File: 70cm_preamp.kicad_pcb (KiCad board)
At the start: 2 copper layers, 33.4 x 13.2 mm, 7 parts, among them J1 RF_IN, J2 RF_OUT, U1 SF2446E, U2 PGA-103+

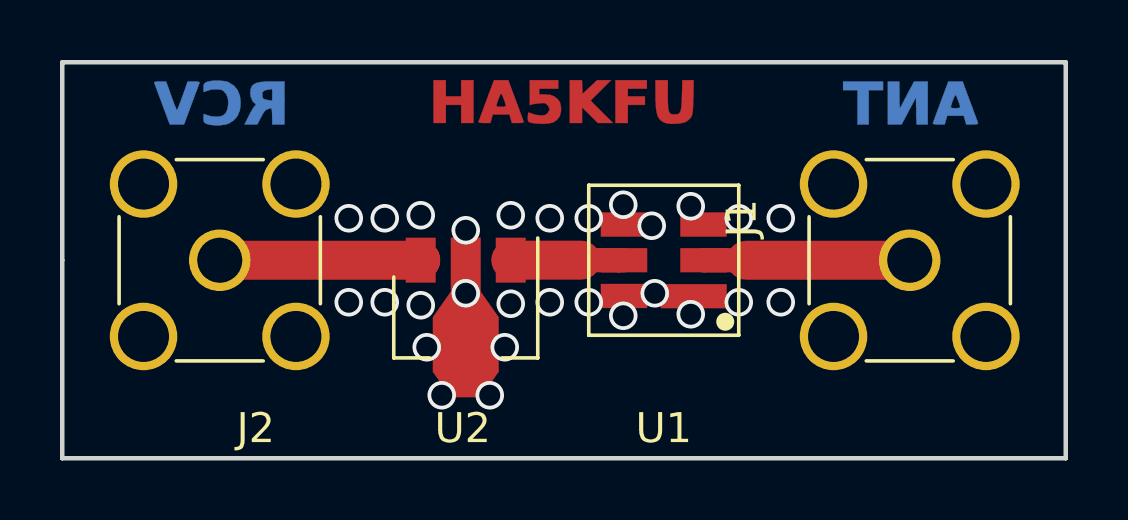
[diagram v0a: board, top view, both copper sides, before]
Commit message: viák
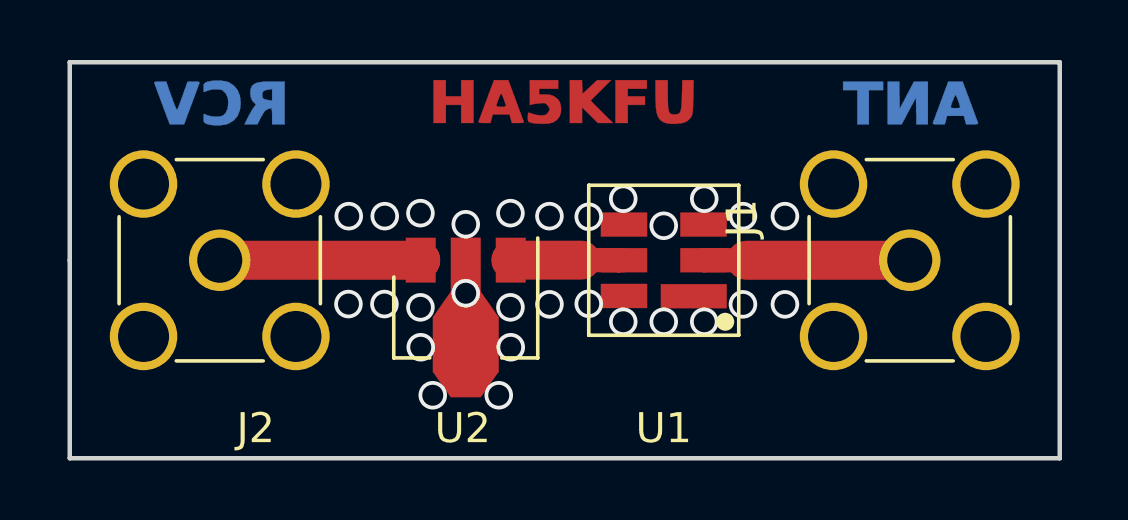
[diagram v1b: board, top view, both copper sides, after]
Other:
- board size 33.4 x 13.2 mm -> 33 x 13.2 mm
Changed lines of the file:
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@@
-(kicad_pcb (version 20171130) (host pcbnew 5.1.6-c6e7f7d~86~ubuntu19.10.1)
+(kicad_pcb (version 20171130) (host pcbnew 5.1.5+dfsg1-2build2)
   (general
     (thickness 1.6)
@@
     )
   )
-  (gr_line (start 42.35 43.4) (end 42.35 36.8) (layer Edge.Cuts) (width 0.15))
-  (gr_line (start 75.8 43.4) (end 42.35 43.4) (layer Edge.Cuts) (width 0.15))
-  (gr_line (start 75.8 30.2) (end 75.8 43.4) (layer Edge.Cuts) (width 0.15))
-  (gr_line (start 42.35 30.2) (end 75.8 30.2) (layer Edge.Cuts) (width 0.15))
-  (gr_line (start 42.35 36.8) (end 42.35 30.2) (layer Edge.Cuts) (width 0.15))
+  (gr_line (start 42.6 43.4) (end 42.6 36.8) (layer Edge.Cuts) (width 0.15))
+  (gr_line (start 75.6 43.4) (end 42.6 43.4) (layer Edge.Cuts) (width 0.15))
+  (gr_line (start 75.6 30.2) (end 75.6 43.4) (layer Edge.Cuts) (width 0.15))
+  (gr_line (start 42.6 30.2) (end 75.6 30.2) (layer Edge.Cuts) (width 0.15))
+  (gr_line (start 42.6 36.8) (end 42.6 30.2) (layer Edge.Cuts) (width 0.15))
   (segment (start 54.2965 36.8) (end 54.3 36.7965) (width 1.3) (layer F.Cu) (net 1))
   (segment (start 47.6 36.8) (end 54.2965 36.8) (width 1.3) (layer F.Cu) (net 1))
-  (via (at 54.3 35.3) (size 0.95) (drill 0.7) (layers F.Cu B.Cu) (net 2))
-  (via (at 53.1 35.4) (size 0.95) (drill 0.7) (layers F.Cu B.Cu) (net 2))
-  (via (at 53.1 38.2) (size 0.95) (drill 0.7) (layers F.Cu B.Cu) (net 2))
-  (via (at 54.3 38.3) (size 0.95) (drill 0.7) (layers F.Cu B.Cu) (net 2))
-  (via (at 57.3 35.3) (size 0.95) (drill 0.7) (layers F.Cu B.Cu) (net 2))
-  (via (at 57.3 38.25) (size 0.95) (drill 0.7) (layers F.Cu B.Cu) (net 2))
-  (via (at 62.1 37.9) (size 0.95) (drill 0.7) (layers F.Cu B.Cu) (net 2))
-  (via (at 62 35.65) (size 0.95) (drill 0.7) (layers F.Cu B.Cu) (net 2))
-  (via (at 63.3 35) (size 0.95) (drill 0.7) (layers F.Cu B.Cu) (net 2))
-  (via (at 63.3 38.6) (size 0.95) (drill 0.7) (layers F.Cu B.Cu) (net 2))
-  (via (at 59.9 38.2) (size 0.95) (drill 0.7) (layers F.Cu B.Cu) (net 2))
-  (via (at 59.9 35.4) (size 0.95) (drill 0.7) (layers F.Cu B.Cu) (net 2))
-  (via (at 58.6 38.2) (size 0.95) (drill 0.7) (layers F.Cu B.Cu) (net 2))
-  (via (at 51.9 38.2) (size 0.95) (drill 0.7) (layers F.Cu B.Cu) (net 2))
-  (via (at 51.9 35.4) (size 0.95) (drill 0.7) (layers F.Cu B.Cu) (net 2))
+  (via (at 54.29 35.23) (size 0.95) (drill 0.7) (layers F.Cu B.Cu) (net 2))
+  (via (at 53.1 35.33) (size 0.95) (drill 0.7) (layers F.Cu B.Cu) (net 2))
+  (via (at 53.09 38.26) (size 0.95) (drill 0.7) (layers F.Cu B.Cu) (net 2))
+  (via (at 54.29 38.37) (size 0.95) (drill 0.7) (layers F.Cu B.Cu) (net 2))
+  (via (at 57.29 35.23) (size 0.95) (drill 0.7) (layers F.Cu B.Cu) (net 2))
+  (via (at 57.29 38.37) (size 0.95) (drill 0.7) (layers F.Cu B.Cu) (net 2))
+  (via (at 62.4 35.65) (size 0.95) (drill 0.7) (layers F.Cu B.Cu) (net 2))
+  (via (at 63.75 34.75) (size 0.95) (drill 0.7) (layers F.Cu B.Cu) (net 2))
+  (via (at 63.75 38.85) (size 0.95) (drill 0.7) (layers F.Cu B.Cu) (net 2))
+  (via (at 59.9 38.25) (size 0.95) (drill 0.7) (layers F.Cu B.Cu) (net 2))
+  (via (at 59.9 35.35) (size 0.95) (drill 0.7) (layers F.Cu B.Cu) (net 2))
+  (via (at 58.59 38.27) (size 0.95) (drill 0.7) (layers F.Cu B.Cu) (net 2))
+  (via (at 51.89 38.26) (size 0.95) (drill 0.7) (layers F.Cu B.Cu) (net 2))
+  (via (at 51.9 35.33) (size 0.95) (drill 0.7) (layers F.Cu B.Cu) (net 2))
   (via (at 55.8 37.9) (size 0.95) (drill 0.7) (layers F.Cu B.Cu) (net 2))
-  (via (at 54.5 39.7) (size 0.95) (drill 0.7) (layers F.Cu B.Cu) (net 2))
-  (via (at 57.1 39.7) (size 0.95) (drill 0.7) (layers F.Cu B.Cu) (net 2))
-  (via (at 55 41.3) (size 0.95) (drill 0.7) (layers F.Cu B.Cu) (net 2))
-  (via (at 56.6 41.3) (size 0.95) (drill 0.7) (layers F.Cu B.Cu) (net 2))
-  (via (at 61.05 38.65) (size 0.95) (drill 0.7) (layers F.Cu B.Cu) (net 2))
-  (via (at 61.05 34.95) (size 0.95) (drill 0.7) (layers F.Cu B.Cu) (net 2))
-  (via (at 55.8 35.8) (size 0.95) (drill 0.7) (layers F.Cu B.Cu) (net 2))
-  (via (at 58.6 35.4) (size 0.95) (drill 0.7) (layers F.Cu B.Cu) (net 2))
-  (via (at 64.9 38.2) (size 0.95) (drill 0.7) (layers F.Cu B.Cu) (net 2))
-  (via (at 64.9 35.4) (size 0.95) (drill 0.7) (layers F.Cu B.Cu) (net 2))
-  (via (at 66.3 35.4) (size 0.95) (drill 0.7) (layers F.Cu B.Cu) (net 2))
-  (via (at 66.3 38.2) (size 0.95) (drill 0.7) (layers F.Cu B.Cu) (net 2))
+  (via (at 54.3 39.7) (size 0.95) (drill 0.7) (layers F.Cu B.Cu) (net 2))
+  (via (at 57.3 39.7) (size 0.95) (drill 0.7) (layers F.Cu B.Cu) (net 2))
+  (via (at 54.7 41.3) (size 0.95) (drill 0.7) (layers F.Cu B.Cu) (net 2))
+  (via (at 56.9 41.3) (size 0.95) (drill 0.7) (layers F.Cu B.Cu) (net 2))
+  (via (at 61.05 38.85) (size 0.95) (drill 0.7) (layers F.Cu B.Cu) (net 2))
+  (via (at 61.05 34.75) (size 0.95) (drill 0.7) (layers F.Cu B.Cu) (net 2))
+  (via (at 55.8 35.6) (size 0.95) (drill 0.7) (layers F.Cu B.Cu) (net 2))
+  (via (at 58.59 35.33) (size 0.95) (drill 0.7) (layers F.Cu B.Cu) (net 2))
+  (via (at 65.04 38.27) (size 0.95) (drill 0.7) (layers F.Cu B.Cu) (net 2))
+  (via (at 65.04 35.33) (size 0.95) (drill 0.7) (layers F.Cu B.Cu) (net 2))
+  (via (at 66.44 35.33) (size 0.95) (drill 0.7) (layers F.Cu B.Cu) (net 2))
+  (via (at 66.44 38.27) (size 0.95) (drill 0.7) (layers F.Cu B.Cu) (net 2))
+  (via (at 62.4 38.85) (size 0.95) (drill 0.7) (layers F.Cu B.Cu) (net 2))
   (segment (start 70.6 36.8) (end 65.15 36.8) (width 1.3) (layer F.Cu) (net 3))
   (segment (start 63.75 36.8) (end 65.15 36.8) (width 0.81) (layer F.Cu) (net 3))
@@
     (polygon
       (pts
-        (xy 75.8 43.4) (xy 42.35 43.4) (xy 42.35 30.2) (xy 75.8 30.2)
+        (xy 75.6 43.4) (xy 42.6 43.4) (xy 42.6 30.2) (xy 75.6 30.2)
       )
     )
@@
     (polygon
       (pts
-        (xy 75.8 43.4) (xy 42.35 43.4) (xy 42.35 30.2) (xy 75.8 30.2)
+        (xy 75.6 43.4) (xy 42.6 43.4) (xy 42.6 30.2) (xy 75.6 30.2)
       )
     )
